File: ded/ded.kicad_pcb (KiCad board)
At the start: 2 copper layers, 10.6 x 15 mm, 3 parts, among them J1 USB_C_Receptacle_PowerOnly_6P, J2 USB_C_Receptacle_PowerOnly_6P

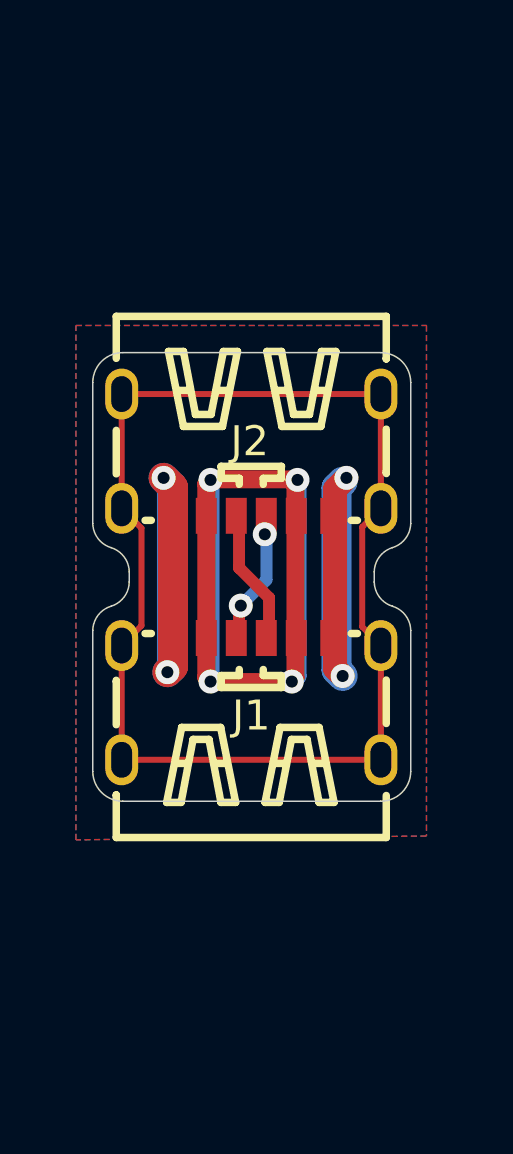
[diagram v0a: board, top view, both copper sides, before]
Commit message: candidate designs for ded and deh couplers
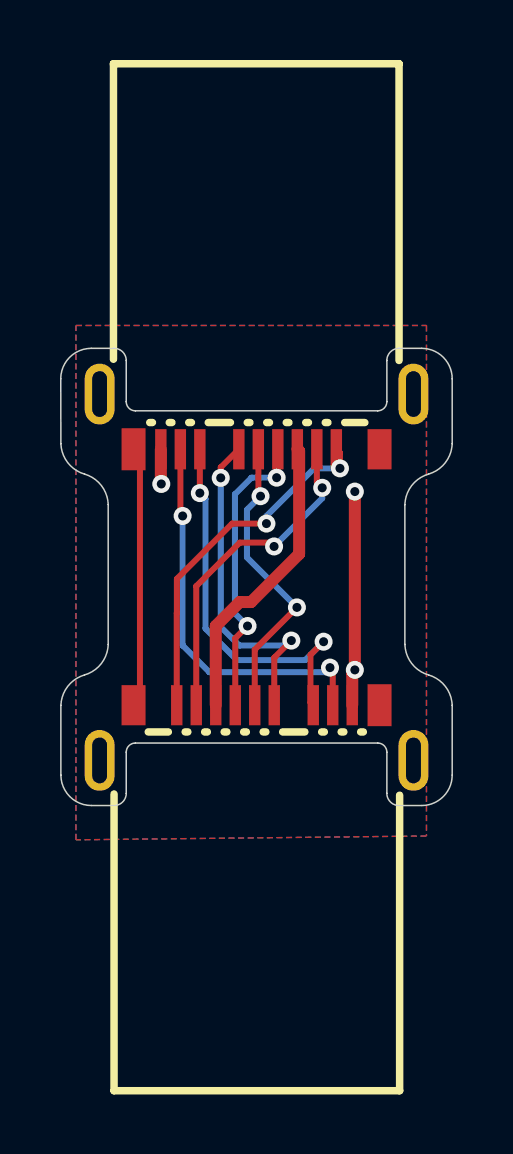
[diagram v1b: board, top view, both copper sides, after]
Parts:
- removed J1, J2: USB_C_Receptacle_PowerOnly_6P, ded:TYPE-C-SMD_TYPE-C-6P_5
- added USB1: GT-USB-8016A, ded:USB-TYPE-C-SMD_GT-USB-8016A, F.Cu at (100.0, 106.3)
- added USB2: GT-USB-8016A, ded:USB-TYPE-C-SMD_GT-USB-8016A, F.Cu at (100.0, 95.9)
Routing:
- net /S1: track 42.7 -> 0.00 mm
- net VBUS: track 32.8 -> 9.93 mm, vias 4 -> 0
- net GND: track 26.9 -> 8.32 mm, vias 4 -> 3
- net Net-(USB1-TX1+): track 0.00 -> 13.2 mm, vias 0 -> 2
- net Net-(USB1-TX1-): track 0.00 -> 13.0 mm, vias 0 -> 2
- net Net-(USB1-RX1-): track 0.00 -> 12.0 mm, vias 0 -> 2
- net Net-(USB1-CC1): track 0.00 -> 11.2 mm, vias 0 -> 2
- net Net-(USB1-RX1+): track 0.00 -> 11.2 mm, vias 0 -> 2
- net Net-(USB1-D+): track 0.00 -> 10.0 mm, vias 0 -> 2
- net Net-(USB1-D-): track 0.00 -> 9.96 mm, vias 0 -> 2
- net (no net): track 0.00 -> 8.71 mm
- net Net-(J1-CC1): track 4.75 -> 0.00 mm, vias 2 -> 0
- net Net-(J1-CC2): track 4.74 -> 0.00 mm
- added copper zone on B.Cu, net GND
- added copper zone on F.Cu, net VBUS
- removed copper zone on F.Cu, net GND
- removed copper zone on B.Cu, net VBUS
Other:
- board size 10.6 x 15 mm -> 13 x 15.2 mm
